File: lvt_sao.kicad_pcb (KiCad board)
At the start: 2 copper layers, 69 x 90.1 mm, 17 parts, among them Q1 MMBT3904, U1 DFR0299, U2 HC-SR501, U3 ESP8266-01/ESP-01, X1 Badgelife_sao_connector_v169b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

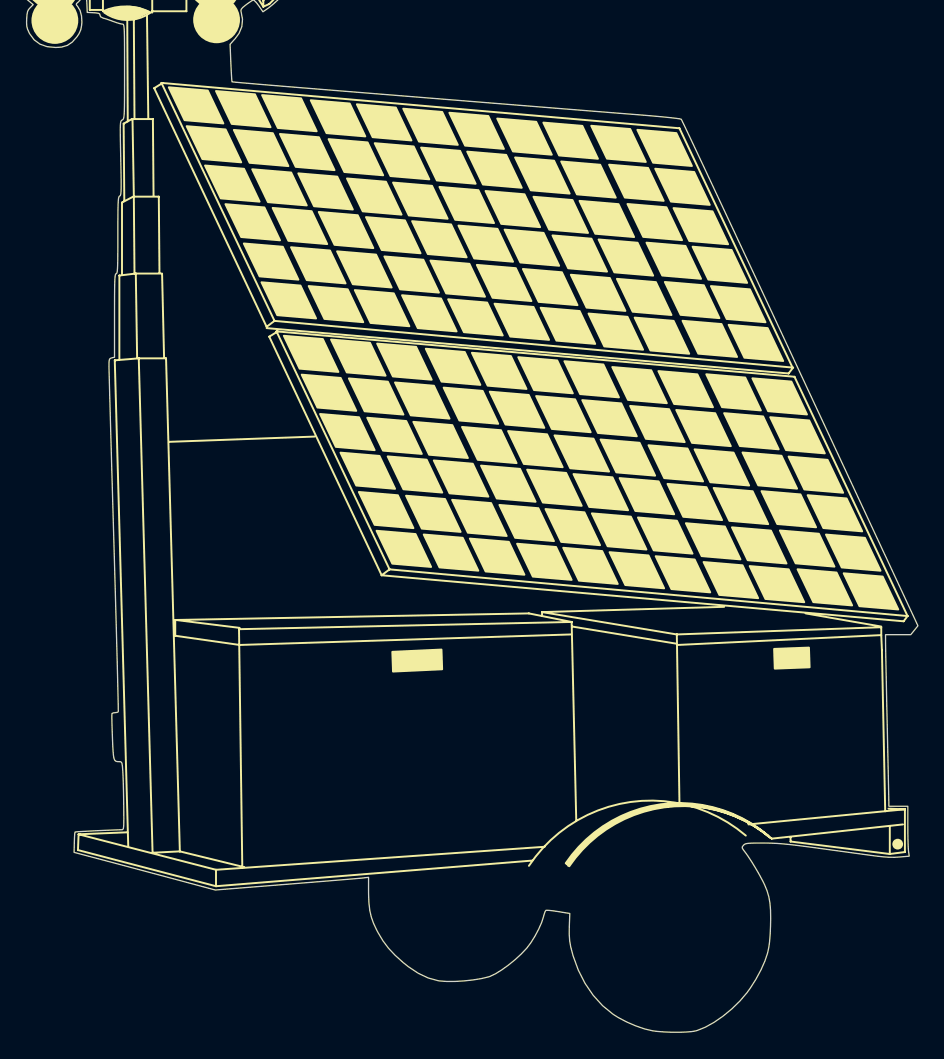
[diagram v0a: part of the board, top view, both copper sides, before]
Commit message: Made it pretty
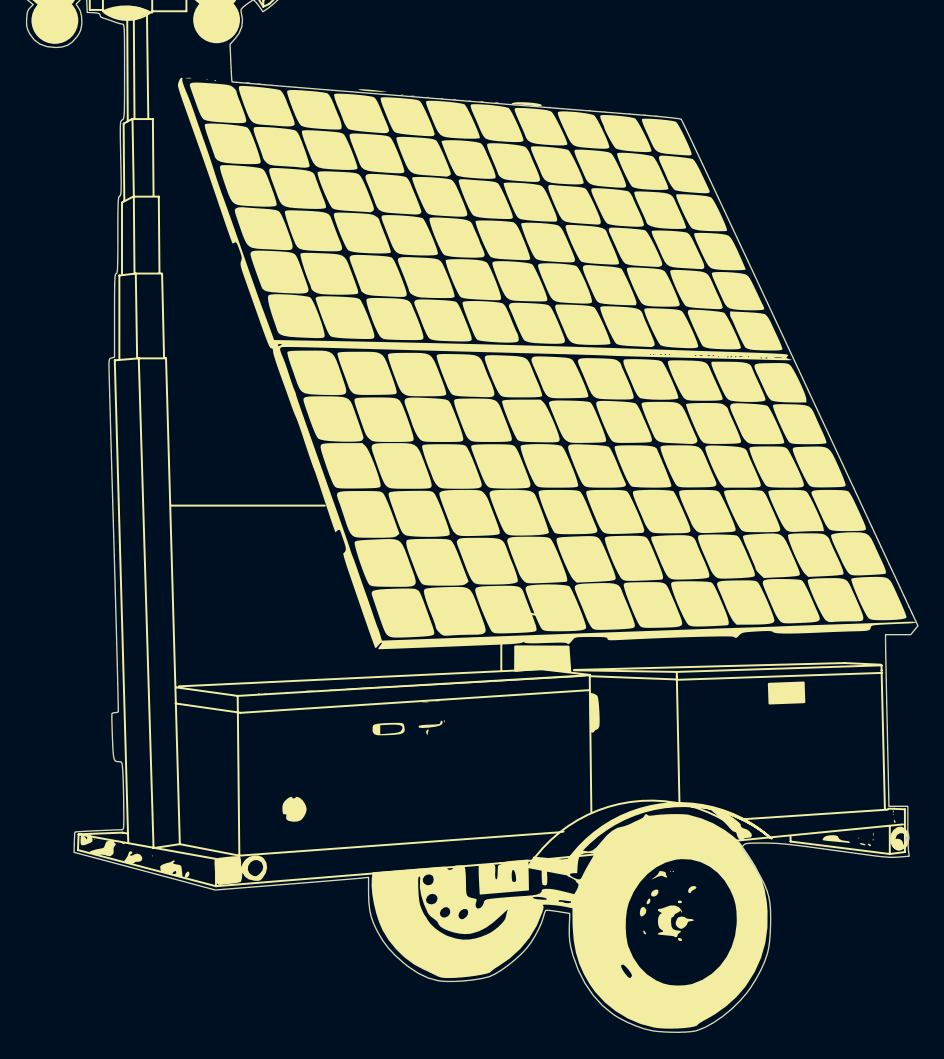
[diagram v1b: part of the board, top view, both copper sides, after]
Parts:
- added G***: LOGO, lvt:trailer_dither, F.Cu at (147.4, 116.6)
